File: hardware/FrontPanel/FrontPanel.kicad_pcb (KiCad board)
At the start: 2 copper layers, 30 x 128.5 mm, 6 parts

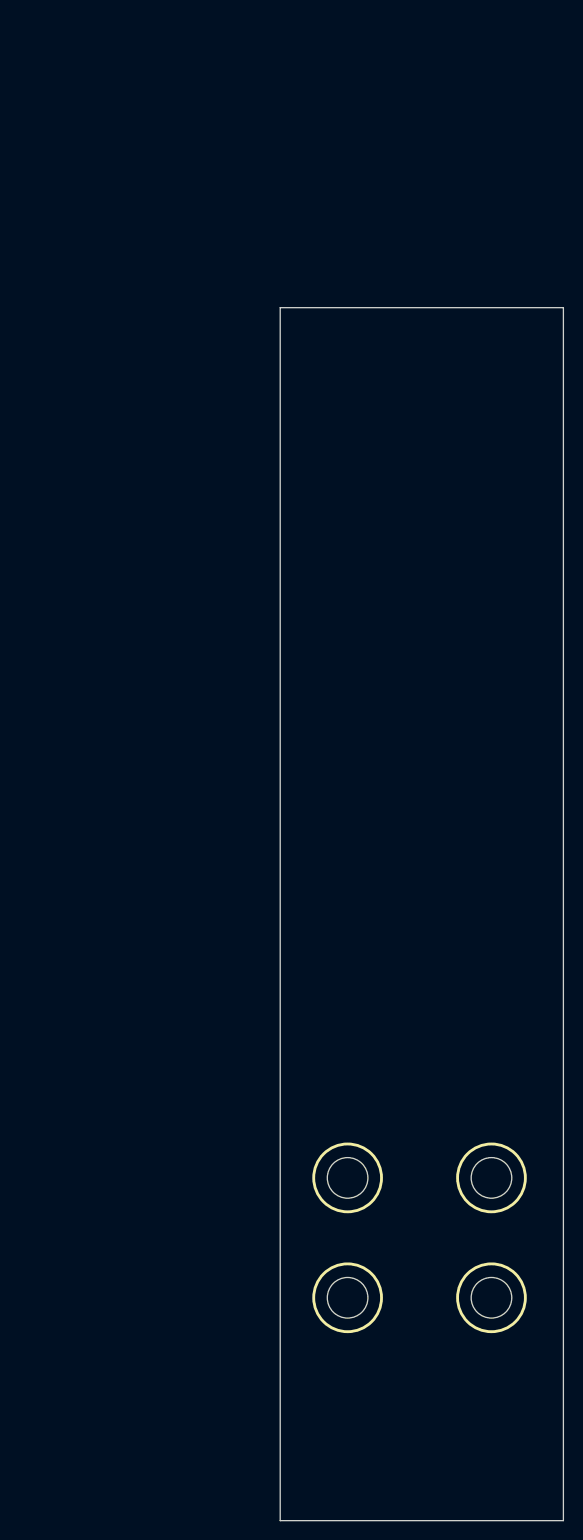
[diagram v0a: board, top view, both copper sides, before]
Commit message: Add latest KICAD updates.
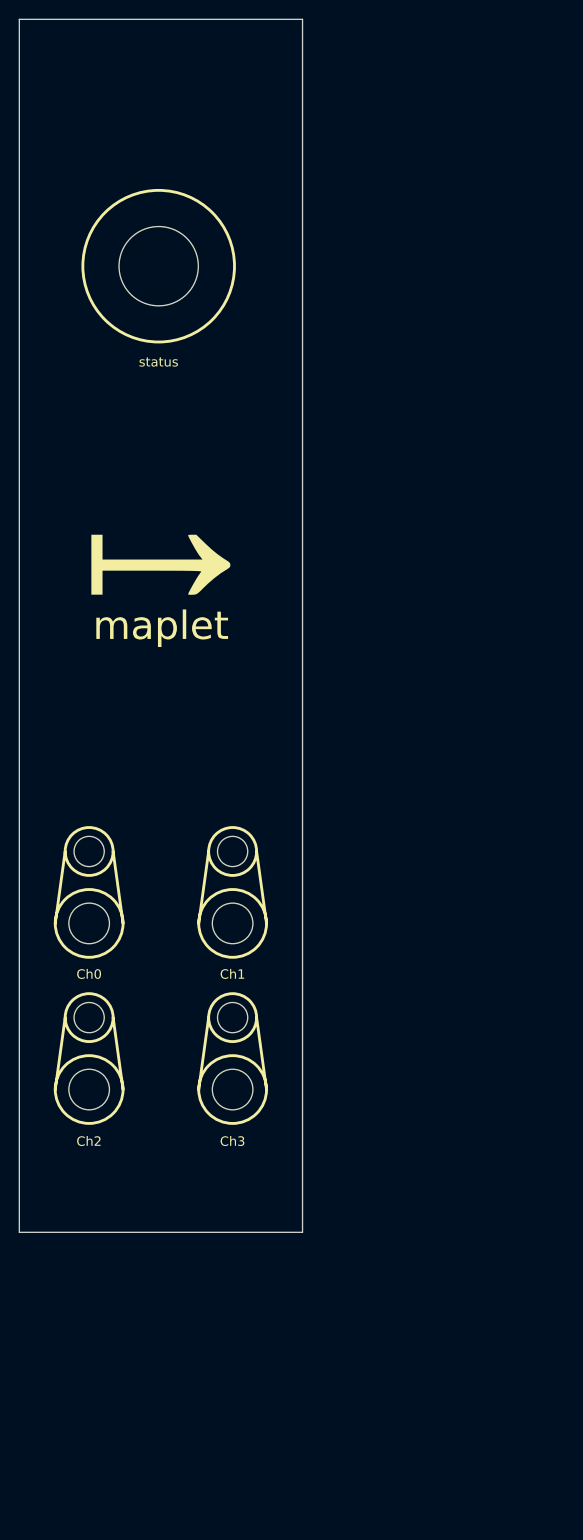
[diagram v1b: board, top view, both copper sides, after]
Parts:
- removed the REF** at (96.5, 162.6)
- removed the REF** at (81.3, 149.9)
- removed the REF** at (96.5, 149.9)
- added Ch0: MountingHole_4.3mm_M4, MountingHole:MountingHole_4.3mm_M4, F.Cu at (53.9, 122.9)
- added Ch1: MountingHole_4.3mm_M4, MountingHole:MountingHole_4.3mm_M4, F.Cu at (69.1, 122.9)
- added Ch3: MountingHole_4.3mm_M4, MountingHole:MountingHole_4.3mm_M4, F.Cu at (69.1, 140.5)
- added G***: LOGO, LOGO, F.Cu at (61.5, 83.8)
- added REF**: MountingHole_3.2mm_M3, MountingHole:MountingHole_3.2mm_M3, F.Cu at (53.9, 132.9)
- added REF**: MountingHole_3.2mm_M3, MountingHole:MountingHole_3.2mm_M3, F.Cu at (53.9, 115.3)
- added REF**: MountingHole_3.2mm_M3, MountingHole:MountingHole_3.2mm_M3, F.Cu at (69.1, 132.9)
- added REF**: MountingHole_3.2mm_M3, MountingHole:MountingHole_3.2mm_M3, F.Cu at (69.1, 115.3)
- added status: MountingHole_8.4mm_M8, MountingHole:MountingHole_8.4mm_M8, F.Cu at (61.3, 53.3)
- moved REF** 41.2 mm to (51.6, 30.1)
- moved REF** 41.2 mm to (51.6, 152.6)
- moved Ch2 35.2 mm to (53.9, 140.5)
- renumbered REF** to Ch2
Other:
- board text added: "maplet"
